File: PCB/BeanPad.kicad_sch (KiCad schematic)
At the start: 9 parts, among them J1 Conn_01x05_Socket, J2 Display, J3 Conn_01x05_Socket, J4 Conn_01x05_Socket, SW1 SW_Push, SW2 SW_Push, SW3 SW_Push, U1 XIAO-RP2040-DIP

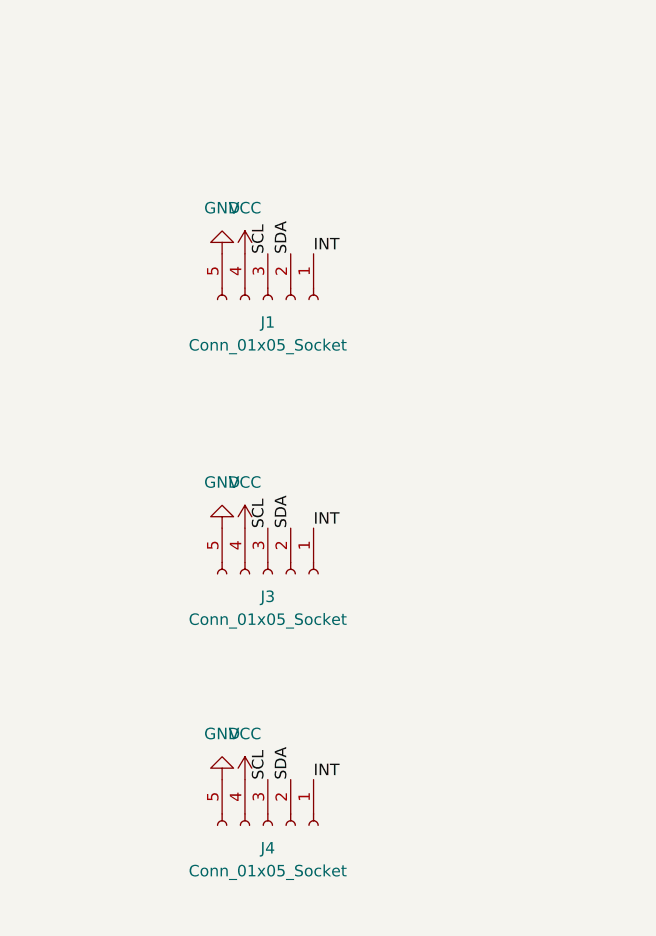
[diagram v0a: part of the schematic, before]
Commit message: PCB finished v1
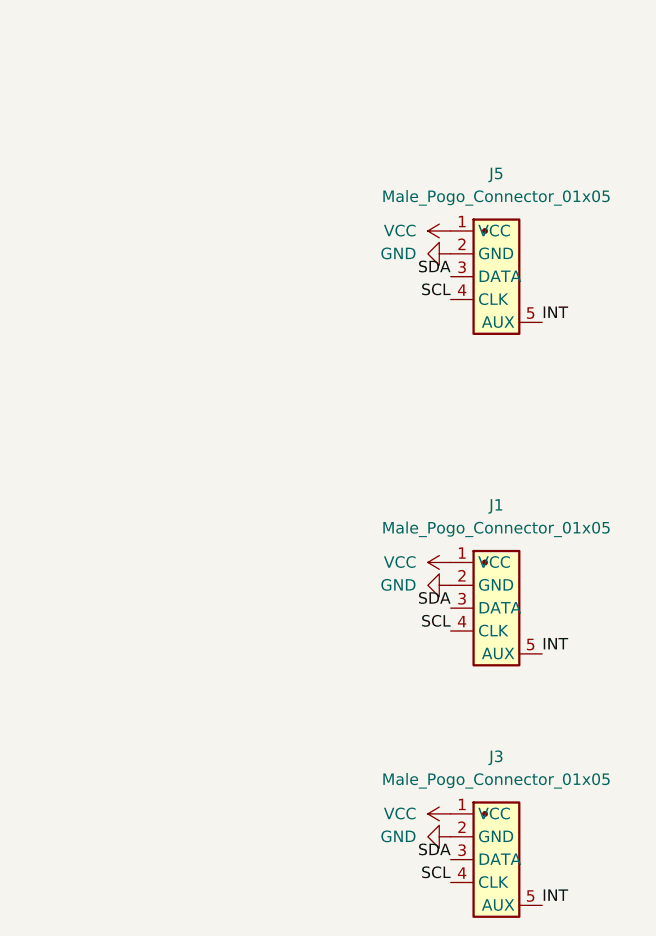
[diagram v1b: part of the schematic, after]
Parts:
- removed J1, J3, J4: Conn_01x05_Socket, Connector_Pogo:male_only_connector, symbol Connector:Conn_01x05_Socket
- added J1, J3, J5: Male_Pogo_Connector_01x05, Conn_Pogo:male_only_connector_5pin_Version3, symbol Conn_Pogo:Male_Pogo_Connector_01x05
- U1: footprint Module:MOUDLE14P-XIAO-DIP-SMD -> Module:XIAO-RP2040-DIP
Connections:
- net GND: now also J1.2 (GND), J3.2 (GND), J5.2 (GND)
- net INT: now also J1.5 (AUX), J3.5 (AUX), J5.5 (AUX)
- net SCL: now also J1.4 (CLK), J3.4 (CLK), J5.4 (CLK)
- net SDA: now also J1.3 (DATA), J3.3 (DATA), J5.3 (DATA)
- net VCC: now also J1.1 (VCC), J3.1 (VCC), J5.1 (VCC)
